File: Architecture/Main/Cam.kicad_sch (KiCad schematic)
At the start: 6 parts, among them J3 Conn_01x03_Pin, J4 Conn_02x09_Odd_Even, U3 74LS04, Y1 Crystal_Small

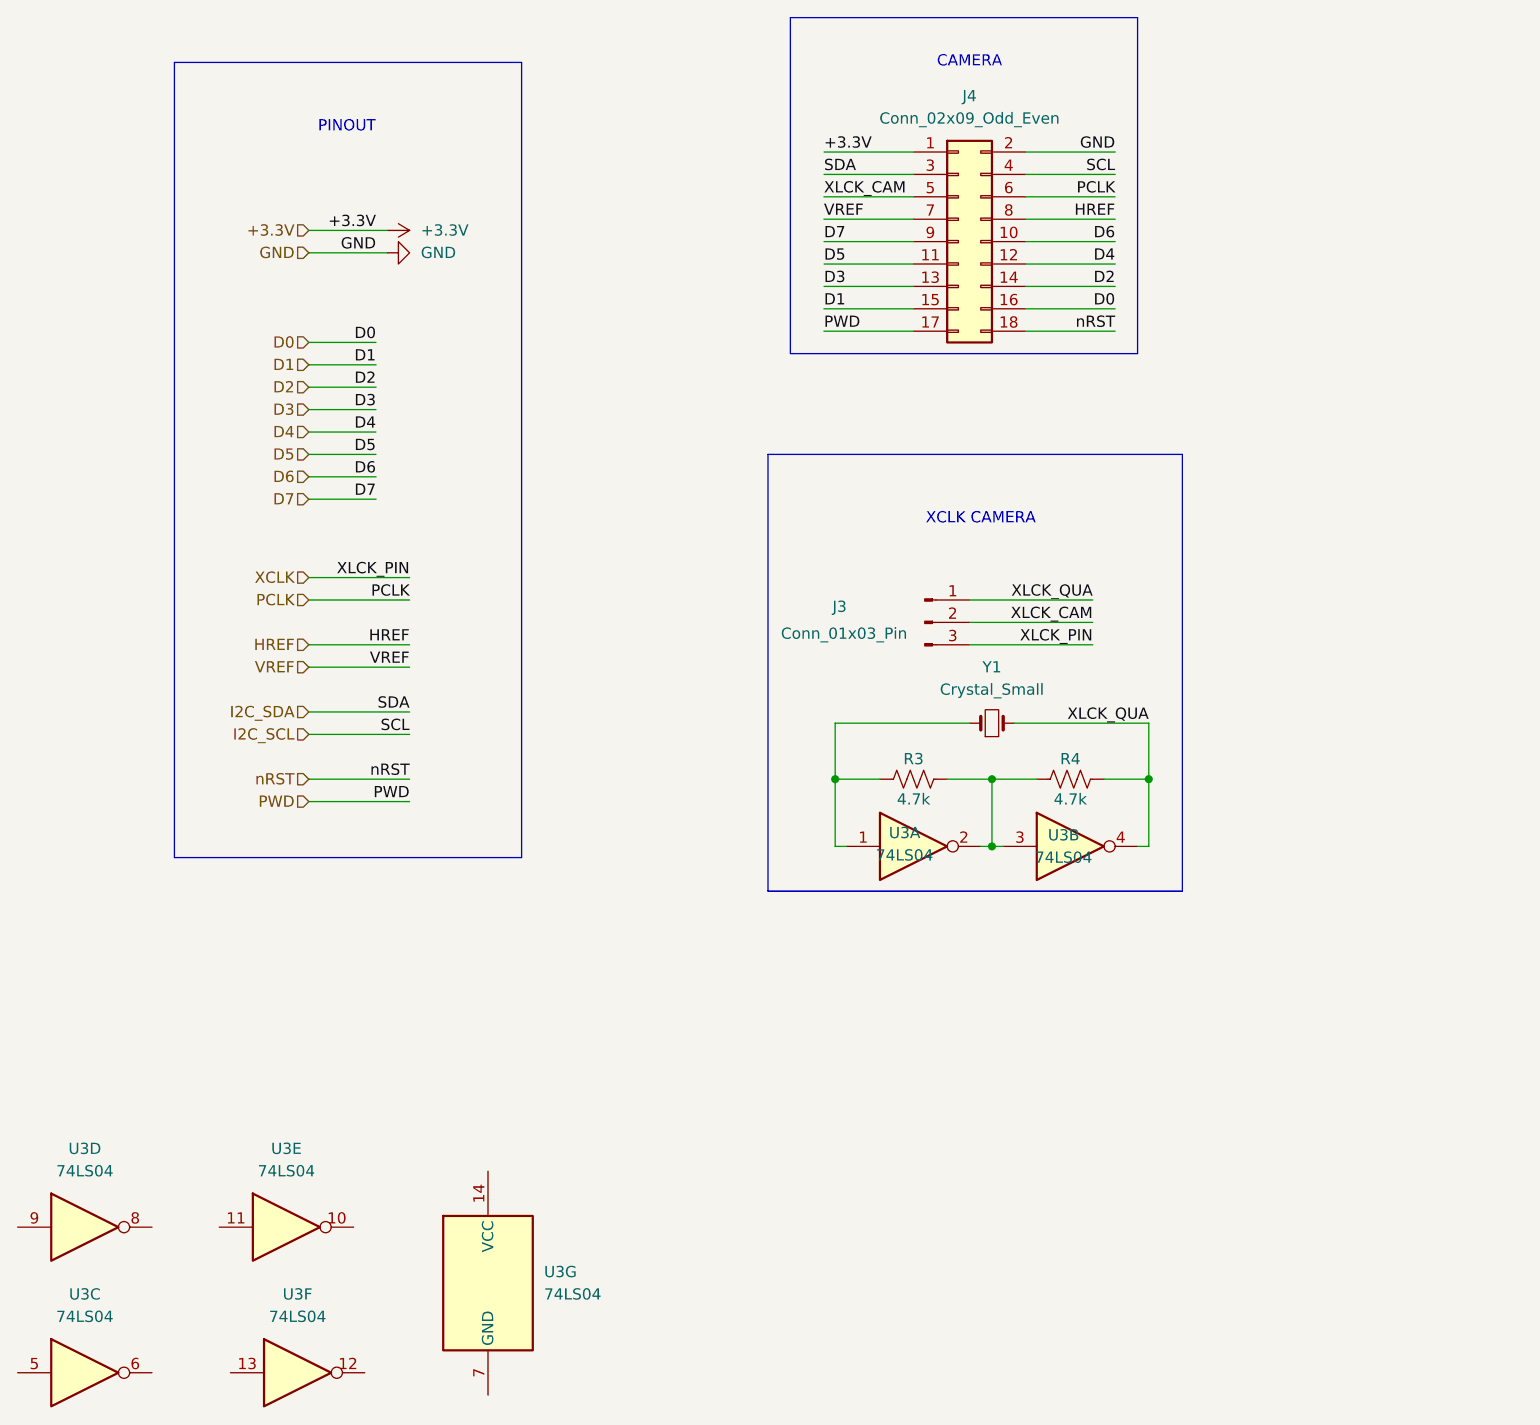
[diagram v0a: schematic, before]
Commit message: Archi_2
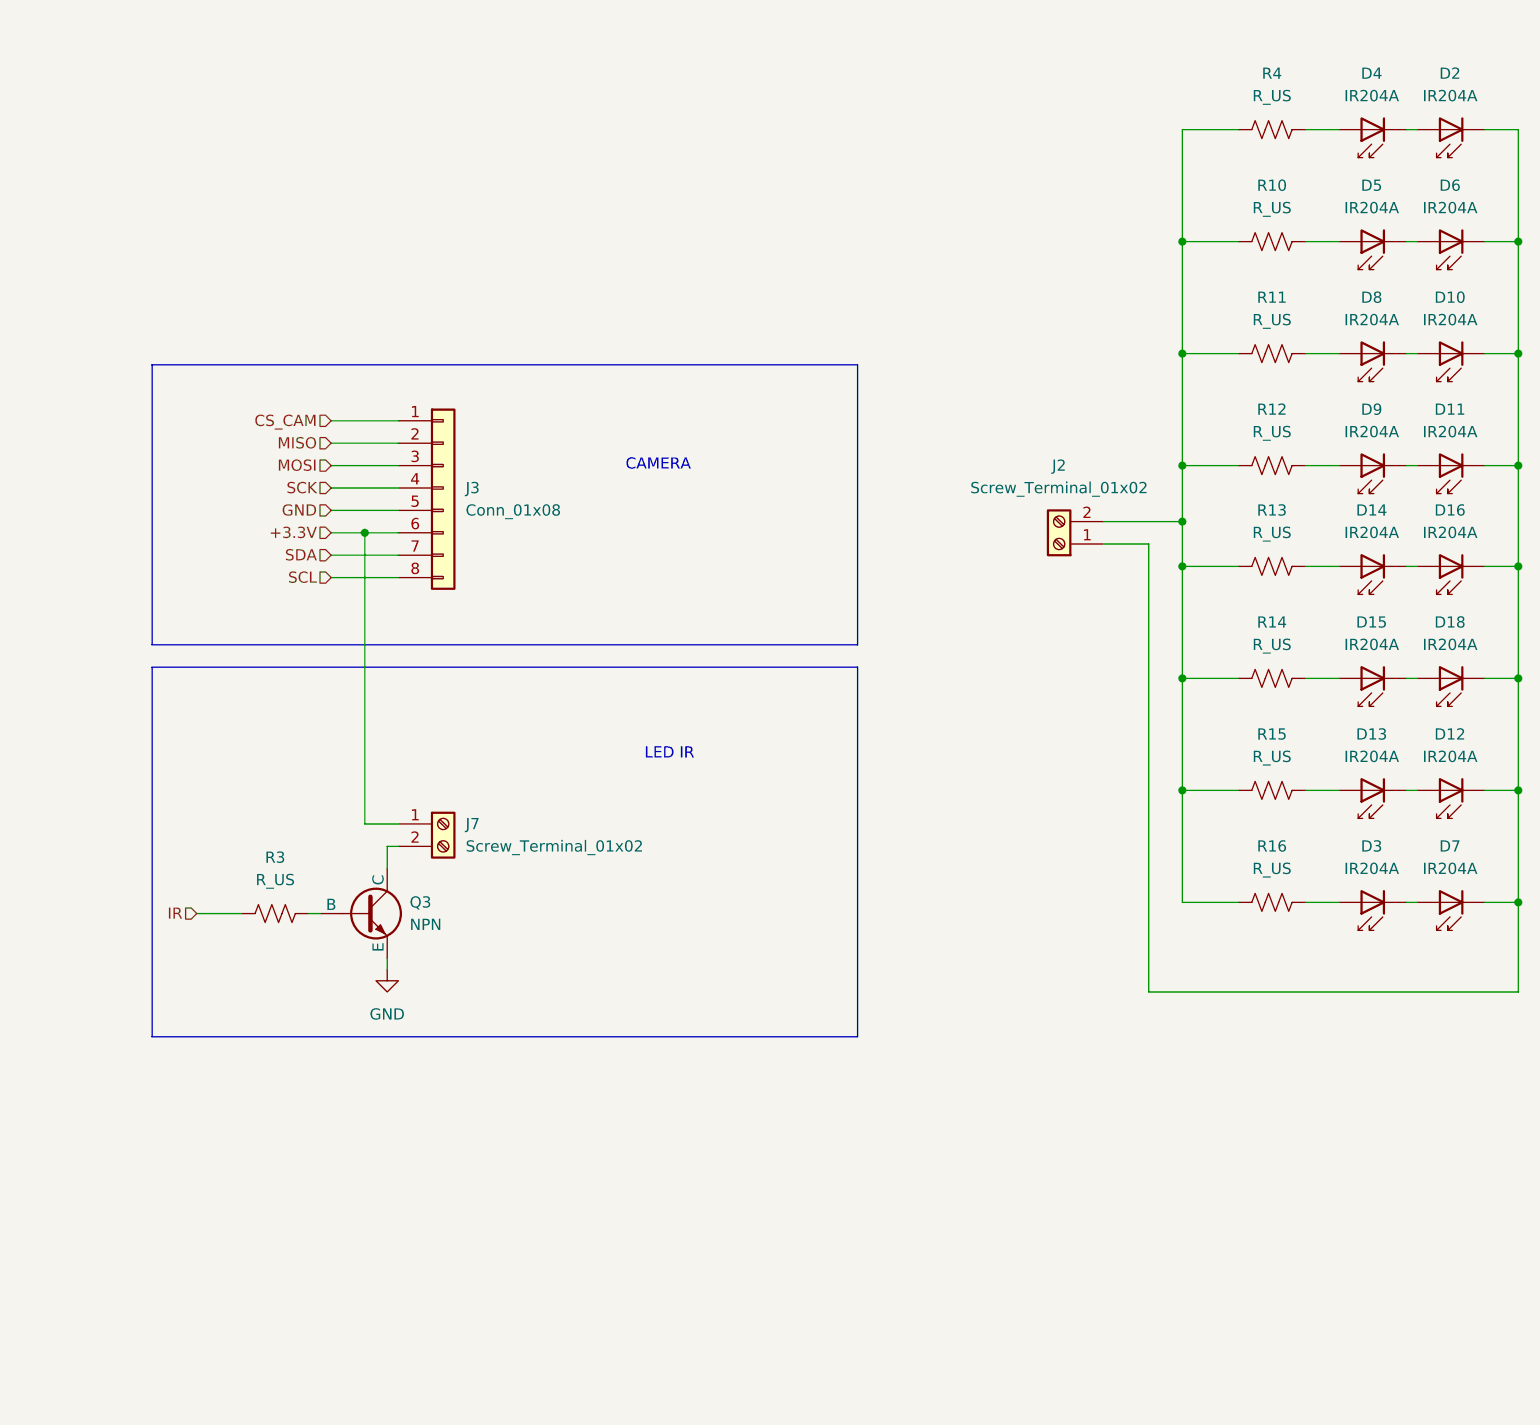
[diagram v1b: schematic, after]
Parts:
- removed J3: Conn_01x03_Pin, symbol Connector:Conn_01x03_Pin
- removed J4: Conn_02x09_Odd_Even, symbol Connector_Generic:Conn_02x09_Odd_Even
- removed U3: 74LS04, symbol 74xx:74LS04
- removed Y1: Crystal_Small, symbol Device:Crystal_Small
- added D10, D11, D12, D13, D14, D15, D16, D18, D2, D3, D4, D5, D6, D7, D8, D9: IR204A, LED_THT:LED_D3.0mm_IRBlack, symbol LED:IR204A
- added J2, J7: Screw_Terminal_01x02, symbol Connector:Screw_Terminal_01x02
- added J3: Conn_01x08, symbol Connector_Generic:Conn_01x08
- added Q3: NPN, symbol Simulation_SPICE:NPN
- added R10, R11, R12, R13, R14, R15, R16: R_US, Resistor_SMD:R_0805_2012Metric_Pad1.20x1.40mm_HandSolder, symbol Device:R_US
- R3, R4: value 4.7k -> R_US
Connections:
- net +3.3V: now also J3.6 (Pin_6), J7.1 (Pin_1)
- net GND: now also J3.5 (Pin_5), Q3.3 (E)
- net at R4.1: now also J2.2 (Pin_2), R10.1, R11.1, R12.1, R13.1, R14.1, R15.1, R16.1; no longer R3.2
- net IR: now reaches R3.1
- net XLCK_QUA: no longer names the net of R4.2
- net XLCK_QUA: now also D4.2 (A)
- new net: D8.2 (A), R11.2
- new net: D5.2 (A), R10.2
- new net: J7.2 (Pin_2), Q3.1 (C)
- new net: D3.2 (A), R16.2
- new net: D2.2 (A), D4.1 (K)
- new net: Q3.2 (B), R3.2
- new net: D5.1 (K), D6.2 (A)
- new net: D15.1 (K), D18.2 (A)
- new net: D15.2 (A), R14.2
- new net: D3.1 (K), D7.2 (A)
- new net: D10.1 (K), D11.1 (K), D12.1 (K), D16.1 (K), D18.1 (K), D2.1 (K), D6.1 (K), D7.1 (K), J2.1 (Pin_1)
- new net: D11.2 (A), D9.1 (K)
- new net: D10.2 (A), D8.1 (K)
- new net: D14.1 (K), D16.2 (A)
- new net: D14.2 (A), R13.2
- new net: D13.2 (A), R15.2
- new net: D9.2 (A), R12.2
- new net: D12.2 (A), D13.1 (K)
- new net CS_CAM: J3.1 (Pin_1)
- new net MISO: J3.2 (Pin_2)
- new net MOSI: J3.3 (Pin_3)
- new net SCK: J3.4 (Pin_4)
- new net SCL: J3.8 (Pin_8)
- new net SDA: J3.7 (Pin_7)
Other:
- note added: "LED IR"
- note removed: "PINOUT"
- note removed: "XCLK CAMERA"
